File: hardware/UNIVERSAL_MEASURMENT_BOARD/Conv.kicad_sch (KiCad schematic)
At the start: 25 parts, among them U10 LMR50410YFQDBVRQ1, U7 LMR50410Y5FQDBVRQ1, U8 RAA2114034GP3#JA0, U9 LMR50410YFQDBVRQ1

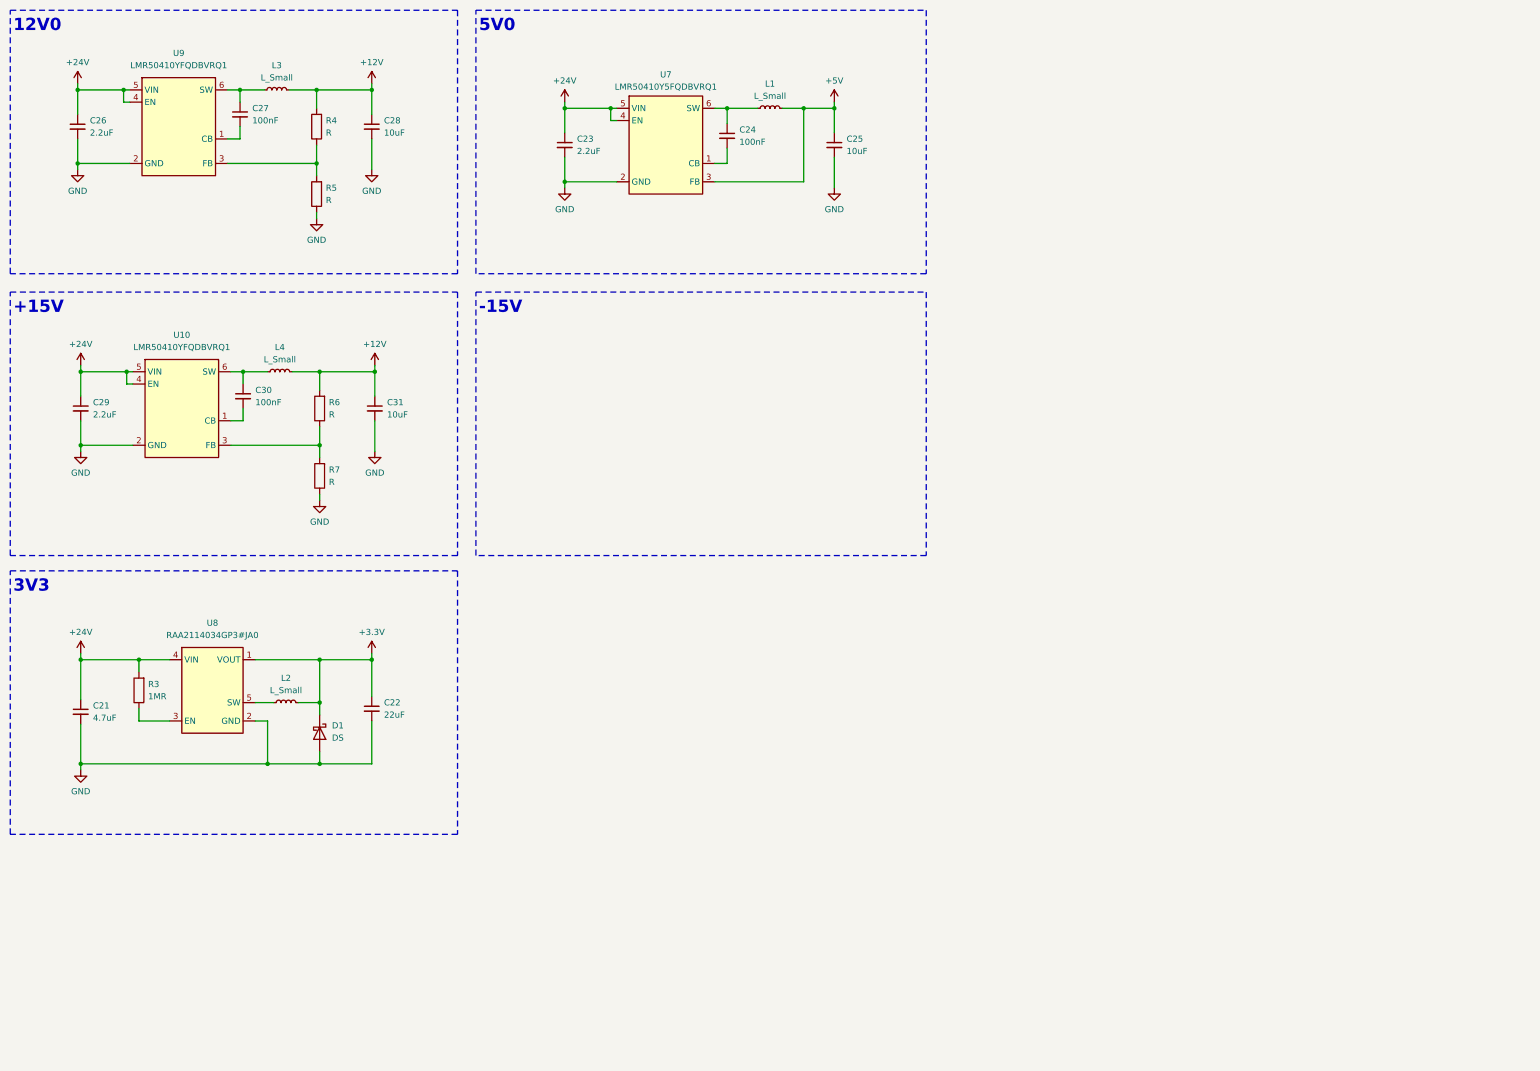
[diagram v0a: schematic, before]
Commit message: continued
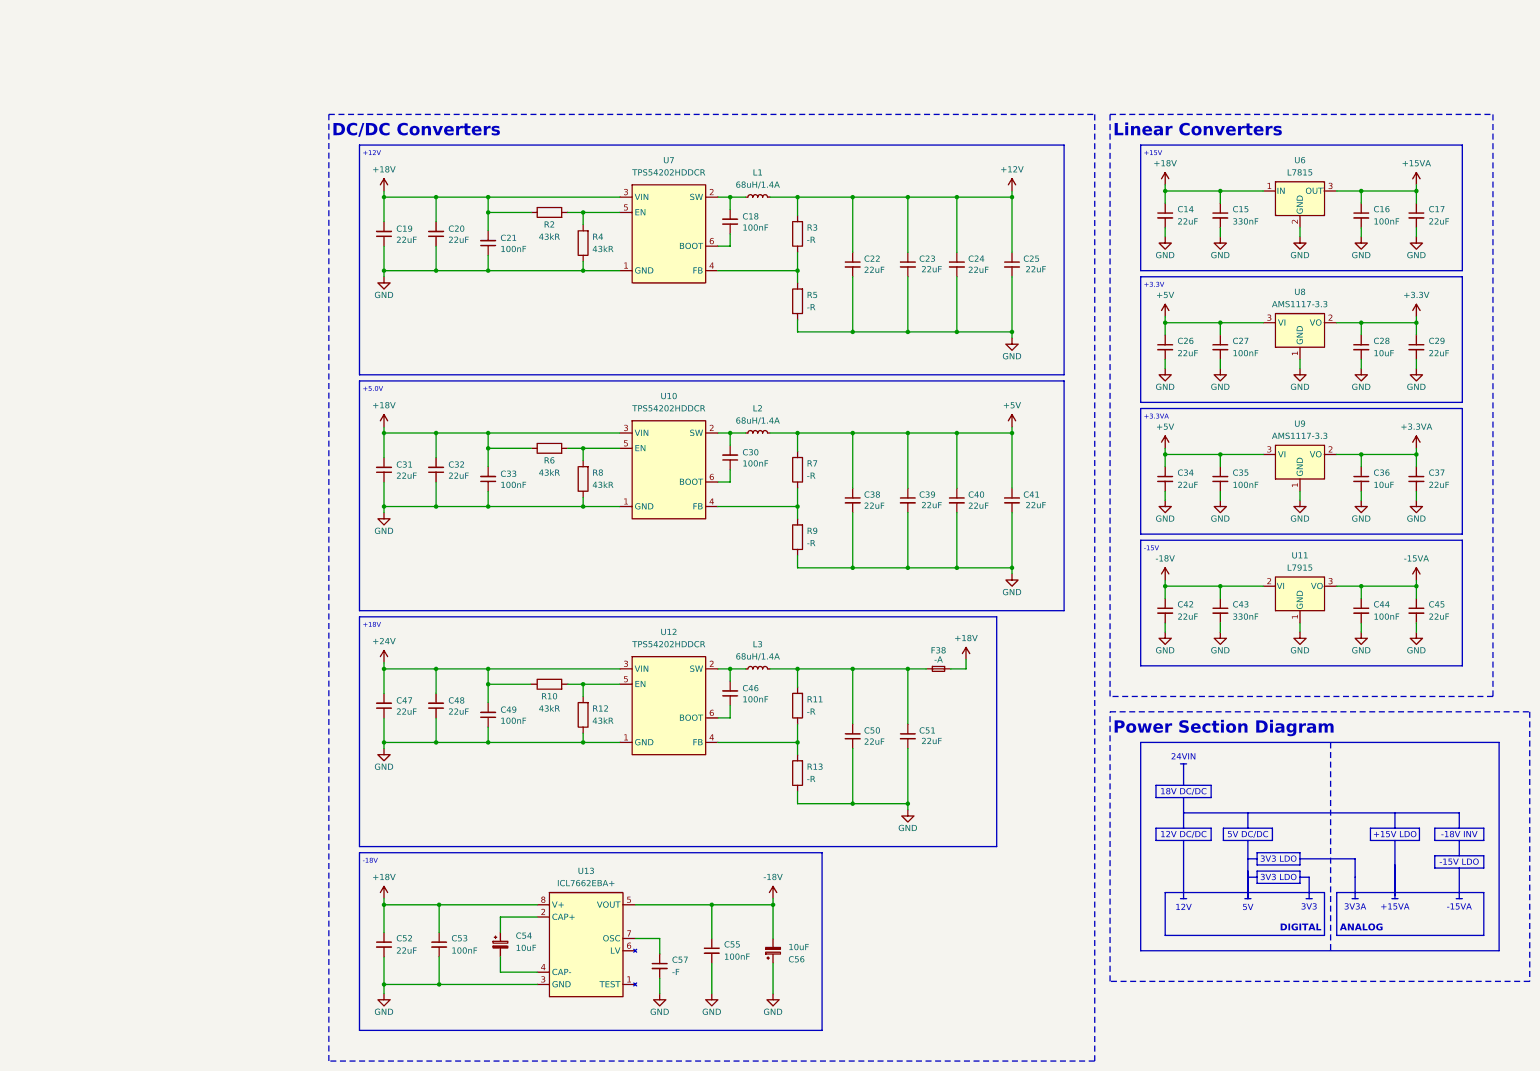
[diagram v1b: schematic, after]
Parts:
- removed D1: DS, symbol Device:D_Schottky
- removed L1, L2, L3, L4: L_Small, symbol Device:L_Small
- removed U10, U9: LMR50410YFQDBVRQ1, SOT95P280X145-6N, symbol LMR50410YFQDBVRQ1:LMR50410YFQDBVRQ1
- removed U7: LMR50410Y5FQDBVRQ1, SOT95P280X145-6N, symbol LMR50410Y5FQDBVRQ1:LMR50410Y5FQDBVRQ1
- removed U8: RAA2114034GP3#JA0, SOT95P280X110-5N, symbol RAA2114034GP3#JA0:RAA2114034GP3#JA0
- added C14, C17, C19, C20, C32, C34, C37, C38, C39, C40, C41, C42, C45, C47, C48, C50, C51, C52: 22uF, Capacitor_SMD:C_0805_2012Metric, symbol Device:C_Small
- added C15, C43: 330nF, Capacitor_SMD:C_0805_2012Metric, symbol Device:C_Small
- added C16, C35, C44, C53, C55: 100nF, Capacitor_SMD:C_0805_2012Metric, symbol Device:C_Small
- added C18, C33, C46, C49: 100nF, Capacitor_SMD:C_0603_1608Metric, symbol Device:C_Small
- added C36: 10uF, Capacitor_SMD:C_0805_2012Metric, symbol Device:C_Small
- added C54, C56: 10uF, symbol Device:C_Polarized_Small
- added C57: -F, Capacitor_SMD:C_0805_2012Metric, symbol Device:C_Small
- added F38: -A, symbol Device:Fuse_Small
- added L1, L2, L3: 68uH/1.4A, Inductor_SMD:L_TDK_VLS6045EX_VLS6045AF, symbol Samacsys_kicad_sym:SRR4028-271Y
- added R10, R12, R2, R8: 43kR, symbol Device:R
- added R11, R13, R9: -R, symbol Device:R
- added U10, U12, U7: TPS54202HDDCR, SOT95P280X110-6N, symbol TPS54202HDDCR:TPS54202HDDCR
- added U11: L7915, symbol Regulator_Linear:L7915
- added U13: ICL7662EBA+, SOIC127P600X175-8N, symbol ICL7662EBA+:ICL7662EBA+
- added U6: L7815, symbol Regulator_Linear:L7815
- added U8, U9: AMS1117-3.3, Package_TO_SOT_SMD:SOT-223-3_TabPin2, symbol Regulator_Linear:AMS1117-3.3
- C21: value 4.7uF -> 100nF; footprint (none) -> Capacitor_SMD:C_0603_1608Metric; Manufacturer_Name (none) -> --; Manufacturer_Part_Number (none) -> C0603C104J3RACTU; Mouser Part Number (none) -> --; Mouser Price/Stock (none) -> https://www.mouser.pl/ProductDetail/KEMET/C0603C104J3RACTU?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
- C22, C27, C28: footprint (none) -> Capacitor_SMD:C_0805_2012Metric; Manufacturer_Name (none) -> MCASH21GCC7684MTCA1J; Manufacturer_Part_Number (none) -> CL21A107MQYNNWE; Mouser Part Number (none) -> 810-C2012X5R1V226MAC
- C23, C26, C29: value 2.2uF -> 22uF; footprint (none) -> Capacitor_SMD:C_0805_2012Metric; Manufacturer_Name (none) -> MCASH21GCC7684MTCA1J; Manufacturer_Part_Number (none) -> CL21A107MQYNNWE; Mouser Part Number (none) -> 810-C2012X5R1V226MAC
- C24: value 100nF -> 22uF; footprint (none) -> Capacitor_SMD:C_0805_2012Metric; Manufacturer_Name (none) -> MCASH21GCC7684MTCA1J; Manufacturer_Part_Number (none) -> CL21A107MQYNNWE; Mouser Part Number (none) -> 810-C2012X5R1V226MAC
- C25, C31: value 10uF -> 22uF; footprint (none) -> Capacitor_SMD:C_0805_2012Metric; Manufacturer_Name (none) -> MCASH21GCC7684MTCA1J; Manufacturer_Part_Number (none) -> CL21A107MQYNNWE; Mouser Part Number (none) -> 810-C2012X5R1V226MAC
- C30: footprint (none) -> Capacitor_SMD:C_0603_1608Metric; Manufacturer_Name (none) -> --; Manufacturer_Part_Number (none) -> C0603C104J3RACTU; Mouser Part Number (none) -> --; Mouser Price/Stock (none) -> https://www.mouser.pl/ProductDetail/KEMET/C0603C104J3RACTU?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
- R3: value 1MR -> -R
- R4, R6: value R -> 43kR
- R5, R7: value R -> -R
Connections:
- net +12V: now also C22.1, C23.1, C24.1, C25.1, R3.2, L1.2; no longer C28.1, C31.1, R4.2, R6.2
- net +24V: now also C47.2, C48.2, C49.2, R10.1, U12.3 (VIN); no longer C21.1, C23.1, C26.1, C29.1, R3.2
- net +3.3V: now also C28.1, C29.1, U8.2 (VO); no longer C22.1
- net +5V: now also C26.1, C27.1, R7.2, C34.1, C35.1, C38.1, C39.1, C40.1, C41.1, L2.2, U8.3 (VI), U9.3 (VI); no longer C25.1
- net GND: now also C21.1, C24.2, C27.2, C31.1, R4.1, C14.2, C15.2, C16.2, C17.2, C19.1, C20.1, C32.1, C33.1, C34.2, C35.2, C36.2, C37.2, C38.2, C39.2, C40.2, C41.2, C42.2, C43.2, C44.2, C45.2, C47.1, C48.1, C49.1, C50.2, C51.2, C52.2, C53.2, C55.2, C56.1, C57.2, R12.1, R13.1, R8.1, R9.1, U10.1 (GND), U11.1 (GND), U12.1 (GND), U13.3 (GND), U6.2 (GND), U7.1 (GND), U8.1 (GND), U9.1 (GND); no longer C21.2, C31.2, R7.1
- net at C30.1: now also U10.6 (BOOT)
- net at C30.2: now also L2.1, U10.2 (SW)
- net +18V: now reaches R6.1
- net +18V: now also C21.2, C31.2, C14.1, C15.1, C19.2, C20.2, C32.2, C33.2, C52.1, C53.1, F38.2, R2.1, U10.3 (VIN), U13.8 (V+), U6.1 (IN), U7.3 (VIN); no longer R7.2
- net at R5.2: now also R3.1, U7.4 (FB); no longer R4.1
- new net: R2.2, R4.2, U7.5 (EN)
- new net: C18.1, U7.6 (BOOT)
- new net: C18.2, L1.1, U7.2 (SW)
- new net: C50.1, C51.1, F38.1, L3.2, R11.2
- new net: R10.2, R12.2, U12.5 (EN)
- new net: C54.1, U13.2 (CAP+)
- new net: C54.2, U13.4 (CAP-)
- new net: R6.2, R8.2, U10.5 (EN)
- new net: R11.1, R13.2, U12.4 (FB)
- new net: R7.1, R9.2, U10.4 (FB)
- new net: C57.1, U13.7 (OSC)
- new net: C46.1, U12.6 (BOOT)
- new net: C46.2, L3.1, U12.2 (SW)
- new net +15VA: C16.1, C17.1, U6.3 (OUT)
- new net +3.3VA: C36.1, C37.1, U9.2 (VO)
- new net -15VA: C44.1, C45.1, U11.3 (VO)
- new net -18V: C42.1, C43.1, C55.1, C56.2, U11.2 (VI), U13.5 (VOUT)
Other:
- note added: "+12V"
- note added: "+15V LDO"
- note added: "+15VA"
- note added: "+18V"
- note added: "+3.3V"
- note added: "+3.3VA"
- note added: "+5.0V"
- note added: "-15V LDO"
- note added: "-15VA"
- note added: "-18V"
- note added: "-18V INV"
- note added: "12V"
- note added: "12V DC/DC"
- note added: "18V DC/DC"
- note added: "24VIN"
- note added: "3V3 LDO"
- note added: "3V3A"
- note added: "5V"
- note added: "5V DC/DC"
- note added: "ANALOG"
- note added: "DC/DC Converters"
- note added: "DIGITAL"
- note added: "Linear Converters"
- note added: "Power Section Diagram"
- note removed: "12V0"
- note removed: "5V0"
- company: (none) -> PUT Motorsport Formula Student team
- title: (none) -> Universal Measurment Board
